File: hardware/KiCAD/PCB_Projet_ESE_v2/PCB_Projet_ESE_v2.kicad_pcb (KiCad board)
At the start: 6 copper layers, 45 x 45 mm, 120 parts, among them J1 Conn_01x06, J10 Conn_ST_STDC14, J2 Conn_01x06, J4 Conn_01x03, J5 Conn_01x04, J6 Conn_01x04, J9 Conn_01x02, SW1 SW_SPST, SW3 SW_SPST, SW4 SW_SPDT, SW5 SW_SPDT, U1 ZXBM5210-SP, U2 ZXBM5210-SP, U3 NCS210, U4 NCS210, U5 STM32G474RETx, U6 ADXL343, Y1 Crystal_GND24_Small

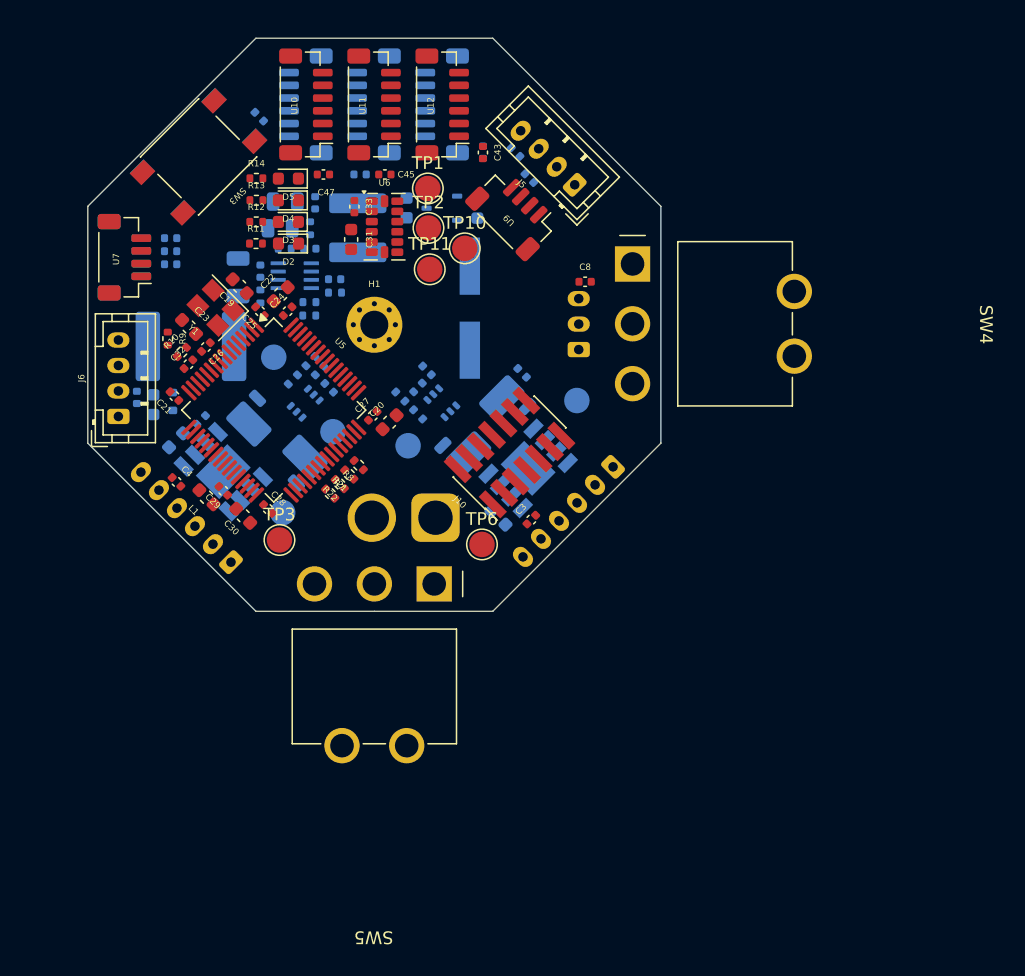
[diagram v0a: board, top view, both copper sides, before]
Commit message: routage en cours
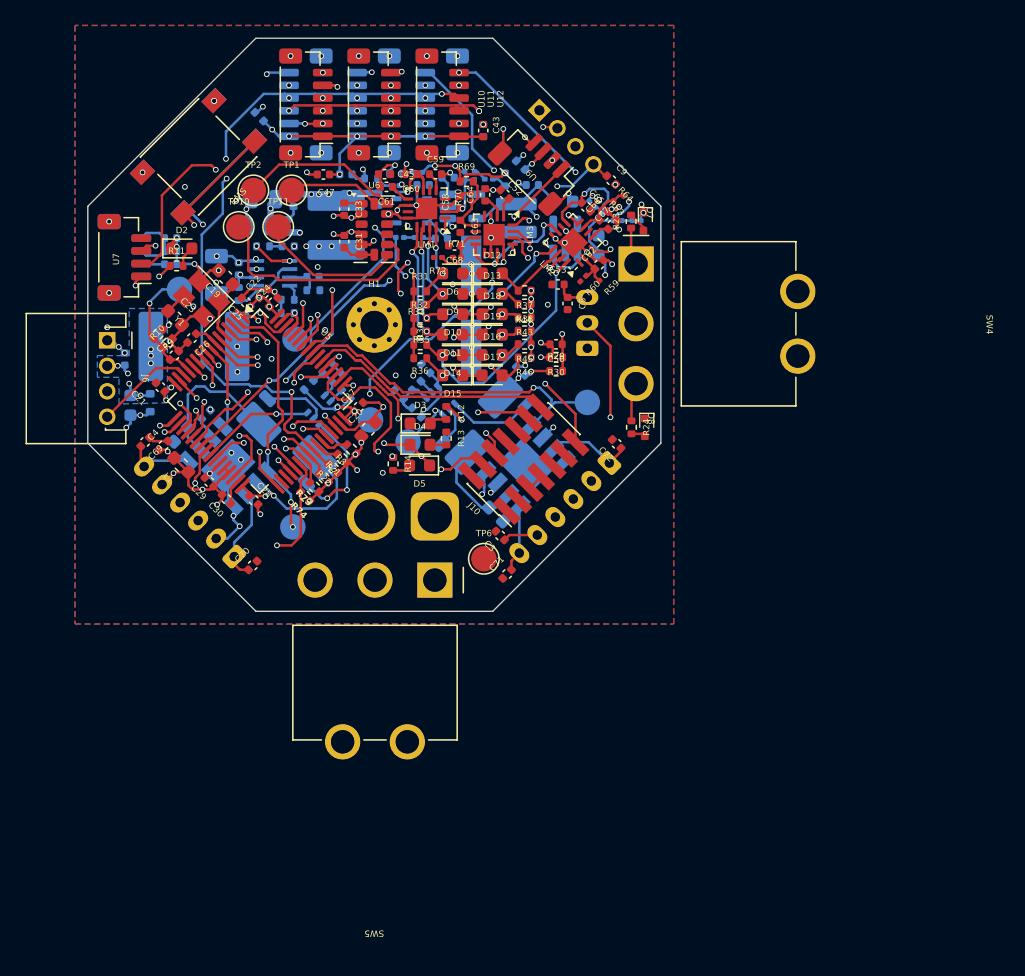
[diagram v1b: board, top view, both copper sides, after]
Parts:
- removed D1: D_TVS_Small, Diode_SMD:D_SOD-523
- added C50: 100n, Capacitor_SMD:C_0402_1005Metric, F.Cu at (91.8, 79.0)
- added C51: 100n, Capacitor_SMD:C_0402_1005Metric, B.Cu at (82.8, 70.7)
- added C52: 100n, Capacitor_SMD:C_0402_1005Metric, F.Cu at (87.7, 67.3)
- added C53: 100n, Capacitor_SMD:C_0402_1005Metric, F.Cu at (91.9, 74.3)
- added C54: 1u, Capacitor_SMD:C_0402_1005Metric, B.Cu at (83.3, 65.9)
- added C55: 1u, Capacitor_SMD:C_0402_1005Metric, B.Cu at (89.9, 66.5)
- added C56: 10u, Capacitor_SMD:C_0603_1608Metric, B.Cu at (92.3, 67.8)
- added C57: 10u, Capacitor_SMD:C_0603_1608Metric, B.Cu at (95.1, 71.3)
- added C58: 100n, Capacitor_SMD:C_0402_1005Metric, F.Cu at (84.2, 67.9)
- added C59: 100n, Capacitor_SMD:C_0402_1005Metric, F.Cu at (82.3, 65.7)
- added C60: 100n, Capacitor_SMD:C_0402_1005Metric, F.Cu at (80.4, 65.7)
- added C61: 100n, Capacitor_SMD:C_0402_1005Metric, F.Cu at (78.5, 66.7)
- added C62: 100n, Capacitor_SMD:C_0402_1005Metric, F.Cu at (95.2, 72.8)
- added C63: 100n, Capacitor_SMD:C_0402_1005Metric, F.Cu at (84.2, 69.8)
- added C64: 100n, Capacitor_SMD:C_0402_1005Metric, F.Cu at (86.2, 67.3)
- added C65: 100n, Capacitor_SMD:C_0402_1005Metric, F.Cu at (94.1, 68.2)
- added C66: 100n, Capacitor_SMD:C_0402_1005Metric, F.Cu at (95.5, 69.0)
- added C67: 100n, Capacitor_SMD:C_0402_1005Metric, F.Cu at (96.2, 69.7)
- added C68: 100n, Capacitor_SMD:C_0402_1005Metric, F.Cu at (83.8, 71.3)
- added C69: 100n, Capacitor_SMD:C_0402_1005Metric, F.Cu at (59.5, 86.7)
- added C70: 100n, Capacitor_SMD:C_0402_1005Metric, F.Cu at (68.0, 96.4)
- added C71: 100n, Capacitor_SMD:C_0402_1005Metric, F.Cu at (87.9, 97.1)
- added C72: 100n, Capacitor_SMD:C_0402_1005Metric, F.Cu at (96.5, 86.8)
- added D10: Yellow LED, LED_SMD:LED_0603_1608Metric, F.Cu at (83.7, 76.7)
- added D11: Yellow LED, LED_SMD:LED_0603_1608Metric, F.Cu at (83.6, 78.3)
- added D12: Orange LED, LED_SMD:LED_0603_1608Metric, F.Cu at (86.8, 73.5)
- added D13: Orange LED, LED_SMD:LED_0603_1608Metric, F.Cu at (86.8, 75.1)
- added D14: Amber LED, LED_SMD:LED_0603_1608Metric, F.Cu at (83.6, 79.9)
- added D15: Amber LED, LED_SMD:LED_0603_1608Metric, F.Cu at (83.7, 81.5)
- added D16: Red LED, LED_SMD:LED_0603_1608Metric, F.Cu at (86.8, 79.9)
- added D17: Red LED, LED_SMD:LED_0603_1608Metric, F.Cu at (86.8, 81.5)
- added D18: Super Red LED, LED_SMD:LED_0603_1608Metric, F.Cu at (86.8, 76.7)
- added D19: Super Red LED, LED_SMD:LED_0603_1608Metric, F.Cu at (86.8, 78.3)
- added D20: ~, Diode_SMD:D_SOD-523, B.Cu at (59.9, 83.6)
- added D6: Green LED, LED_SMD:LED_0603_1608Metric, F.Cu at (83.7, 73.5)
- added D7: YELLOW_LED, mylib:wurth_155060YS75300, F.Cu at (98.6, 68.7)
- added D8: YELLOW_LED, mylib:wurth_155060YS75300, F.Cu at (98.7, 84.9)
- added D9: Green LED, LED_SMD:LED_0603_1608Metric, F.Cu at (83.7, 75.1)
- added L3: 4u7, mylib:WE-TPC-744028004, B.Cu at (88.7, 68.0)
- added LM1: ~, Package_DFN_QFN:WQFN-16-1EP_3x3mm_P0.5mm_EP1.68x1.68mm, F.Cu at (81.6, 68.4)
- added LM2: ~, Package_DFN_QFN:WQFN-16-1EP_3x3mm_P0.5mm_EP1.68x1.68mm, F.Cu at (93.1, 71.1)
- added LM3: ~, Package_DFN_QFN:WQFN-16-1EP_3x3mm_P0.5mm_EP1.68x1.68mm, F.Cu at (86.9, 70.4)
- added R23: 300, Resistor_SMD:R_0402_1005Metric, F.Cu at (97.7, 69.4)
- added R24: 300, Resistor_SMD:R_0402_1005Metric, F.Cu at (97.7, 85.6)
- added R29: 48k7, Resistor_SMD:R_0402_1005Metric, F.Cu at (91.8, 81.1)
- added R30: 39k2, Resistor_SMD:R_0402_1005Metric, F.Cu at (91.8, 80.1)
- added R31: 3k3, Resistor_SMD:R_0402_1005Metric, F.Cu at (81.1, 74.9)
- added R32: 3k3, Resistor_SMD:R_0402_1005Metric, F.Cu at (81.1, 75.9)
- added R33: 1k6, Resistor_SMD:R_0402_1005Metric, F.Cu at (81.1, 77.0)
- added R34: 1k6, Resistor_SMD:R_0402_1005Metric, F.Cu at (81.1, 78.0)
- added R35: 2k, Resistor_SMD:R_0402_1005Metric, F.Cu at (81.1, 79.1)
- added R36: 2k, Resistor_SMD:R_0402_1005Metric, F.Cu at (81.1, 80.1)
- added R37: 1k, Resistor_SMD:R_0402_1005Metric, F.Cu at (89.3, 74.8)
- added R38: 1k, Resistor_SMD:R_0402_1005Metric, F.Cu at (89.3, 75.9)
- added R43: 1k3, Resistor_SMD:R_0402_1005Metric, F.Cu at (89.3, 76.9)
- added R44: 1k3, Resistor_SMD:R_0402_1005Metric, F.Cu at (89.3, 78.0)
- added R45: 2k4, Resistor_SMD:R_0402_1005Metric, F.Cu at (89.3, 79.0)
- added R46: 2k4, Resistor_SMD:R_0402_1005Metric, F.Cu at (89.3, 80.1)
- added R51: 5k23, Resistor_SMD:R_0201_0603Metric, B.Cu at (84.6, 65.8)
- added R52: 100k, Resistor_SMD:R_0201_0603Metric, B.Cu at (85.4, 65.8)
- added R53: 11k, Resistor_SMD:R_0201_0603Metric, B.Cu at (81.0, 65.5)
- added R54: 98k8, Resistor_SMD:R_0402_1005Metric, B.Cu at (79.2, 65.6)
- added R55: 20k, Resistor_SMD:R_0201_0603Metric, B.Cu at (79.2, 66.6)
- added R56: 79k6, Resistor_SMD:R_0402_1005Metric, B.Cu at (77.2, 66.0)
- added R57: 20k, Resistor_SMD:R_0201_0603Metric, B.Cu at (79.5, 70.6)
- added R58: 46k4, Resistor_SMD:R_0201_0603Metric, B.Cu at (81.0, 70.6)
- added R59: 20k, Resistor_SMD:R_0201_0603Metric, F.Cu at (95.4, 73.8)
- added R60: 30k, Resistor_SMD:R_0201_0603Metric, F.Cu at (93.9, 73.9)
- added R61: 47k, Resistor_SMD:R_0201_0603Metric, B.Cu at (96.6, 69.3)
- added R62: 47k, Resistor_SMD:R_0201_0603Metric, B.Cu at (98.1, 69.3)
- added R63: 30k, Resistor_SMD:R_0201_0603Metric, F.Cu at (97.3, 67.6)
- added R64: 20k, Resistor_SMD:R_0201_0603Metric, F.Cu at (96.5, 68.0)
- added R65: 46.4k, Resistor_SMD:R_0201_0603Metric, B.Cu at (95.2, 69.0)
- added R66: 20k, Resistor_SMD:R_0201_0603Metric, B.Cu at (94.6, 68.0)
- added R67: 79k6, Resistor_SMD:R_0402_1005Metric, B.Cu at (87.8, 66.1)
- added R68: 20k, Resistor_SMD:R_0201_0603Metric, B.Cu at (86.5, 66.1)
- added R69: 98k8, Resistor_SMD:R_0402_1005Metric, F.Cu at (84.7, 66.3)
- added R70: 11k, Resistor_SMD:R_0201_0603Metric, F.Cu at (85.2, 67.5)
- added R71: 100k, Resistor_SMD:R_0201_0603Metric, F.Cu at (84.0, 72.2)
- added R72: 5k23, Resistor_SMD:R_0201_0603Metric, F.Cu at (82.5, 72.2)
- added R73: 4k7, Resistor_SMD:R_0402_1005Metric, F.Cu at (72.8, 90.2)
- added R74: 4k7, Resistor_SMD:R_0402_1005Metric, F.Cu at (72.1, 91.0)
- added TP12: ~, Package_TO_SOT_SMD:SOT-23-5, B.Cu at (92.5, 70.7)
- added U16: MCP1802x-xx02xOT, Package_TO_SOT_SMD:SOT-23-5, B.Cu at (84.4, 68.2)
- C22, C30, C31, C41, C42: footprint Capacitor_SMD:C_0603_1608Metric -> Capacitor_SMD:C_0402_1005Metric
- C9: moved to F.Cu
- J5: footprint Connector_JST:JST_PH_B4B-PH-K_1x04_P2.00mm_Vertical -> Connector_THT_Wurth:J_Wurth_WR-WTB_62000411722; moved to B.Cu
- J6: footprint Connector_JST:JST_PH_B4B-PH-K_1x04_P2.00mm_Vertical -> Connector_THT_Wurth:J_Wurth_WR-WTB_62000411722
- R10: value 5k6 -> 16k
- R11: value 240 -> 39
- R12: value 2k9 -> 2k7
- R13: value 1k65 -> 1k6
- R14: value 800 -> 820
- R9: value 20k -> 56k
- TP3: moved to B.Cu
- moved R14 24.9 mm to (79.0, 88.4), turned to -90 degrees
- moved D5 24.8 mm to (81.0, 88.5)
- moved R13 23.9 mm to (83.2, 86.4), turned to -90 degrees
- moved D4 21.8 mm to (81.1, 86.9), turned to 0 degrees
- moved TP3 21.2 mm to (62.2, 74.7), turned to 180 degrees
- moved R12 21.2 mm to (83.2, 84.4), turned to -90 degrees
- moved D3 18.9 mm to (81.1, 85.2), turned to 0 degrees
- moved TP10 17.8 mm to (66.8, 69.8)
- moved TP2 14.1 mm to (68.0, 67.0)
- moved TP11 12.4 mm to (70.0, 69.8)
- moved TP1 10.7 mm to (71.0, 67.0)
- moved TP9 9.06 mm to (77.2, 85.0)
- moved D2 8.39 mm to (62.4, 71.5), turned to 0 degrees
- moved TP5 7.87 mm to (71.3, 78.6)
- moved C9 7.83 mm to (96.1, 66.2)
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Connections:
- SW4 pad G1: (no net) -> unconnected-(SW4-PadG1)
- SW4 pad G2: (no net) -> unconnected-(SW4-PadG2)
- SW5 pad G1: (no net) -> unconnected-(SW5-PadG1)
- SW5 pad G2: (no net) -> unconnected-(SW5-PadG2)
- U5 pad 19: TOF_1_XSHUT -> TOF_4_XSHUT
- U5 pad 21: TOF_2_XSHUT -> TOF_3_XSHUT
- U5 pad 23: TOF_4_XSHUT -> TOF_5_XSHUT
- U5 pad 33: TOF_5_XSHUT -> TOF_2_XSHUT
- U5 pad 38: TOF_SCL -> AMPLI_SCL
- U5 pad 39: TOF_SDA -> AMPLI_SDA
- U5 pad 40: AMPLI_SCL -> TOF_SCL
- U5 pad 41: AMPLI_SDA -> TOF_SDA
- U5 pad 44: TOF_3_XSHUT -> TOF_1_XSHUT
- U5 pad 59: TOF_3_GPIO -> TOF_5_GPIO
- U5 pad 60: TOF_4_GPIO -> TOF_3_GPIO
- U5 pad 61: unconnected-(U5-PB8-Pad61) -> GND
- U5 pad 62: TOF_5_GPIO -> TOF_4_GPIO
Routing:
- net GND: track 0.00 -> 147.2 mm, vias 0 -> 104
- net +3.3V: track 0.00 -> 76.3 mm, vias 0 -> 26
- net TOF_SCL: track 0.00 -> 59.5 mm, vias 0 -> 11
- net TOF_SDA: track 0.00 -> 57.7 mm, vias 0 -> 9
- net NRST: track 0.00 -> 54.5 mm, vias 0 -> 3
- net +5V: track 0.00 -> 50.5 mm, vias 0 -> 21
- net TOF_6_XSHUT: track 0.00 -> 47.5 mm, vias 0 -> 4
- net TOF_1_XSHUT: track 0.00 -> 47.3 mm, vias 0 -> 5
- net Mode_1: track 0.00 -> 45.7 mm, vias 0 -> 1
- net AMPLI_SDA: track 0.00 -> 44.5 mm, vias 0 -> 2
- net TOF_2_XSHUT: track 0.00 -> 43.2 mm, vias 0 -> 5
- net Mode_2: track 0.00 -> 39.9 mm, vias 0 -> 1
- net UART_LIDAR_TX_HD: track 0.00 -> 39.8 mm, vias 0 -> 2
- net PWM_LED: track 0.00 -> 37.2 mm, vias 0 -> 2
- net TOF_5_XSHUT: track 0.00 -> 37.2 mm, vias 0 -> 3
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- added copper zone on In3.Cu, net +3.3V
- added copper zone on In3.Cu, net +5V
- added copper zone on In3.Cu, net +7.4V
- added copper zone on B.Cu, net /5V_Rpi
- added copper zone on B.Cu, net GND
- added copper zone on F.Cu, net GND
- added copper zone on In1.Cu, net GND
- added copper zone on In2.Cu, net GND
- added copper zone on In4.Cu, net GND
- added copper zone on In3.Cu, net IN+
- added copper zone on In3.Cu, net Net-(J9-Pin_2)
